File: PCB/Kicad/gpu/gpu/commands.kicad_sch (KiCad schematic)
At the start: 1 part, among them U1 74LS08

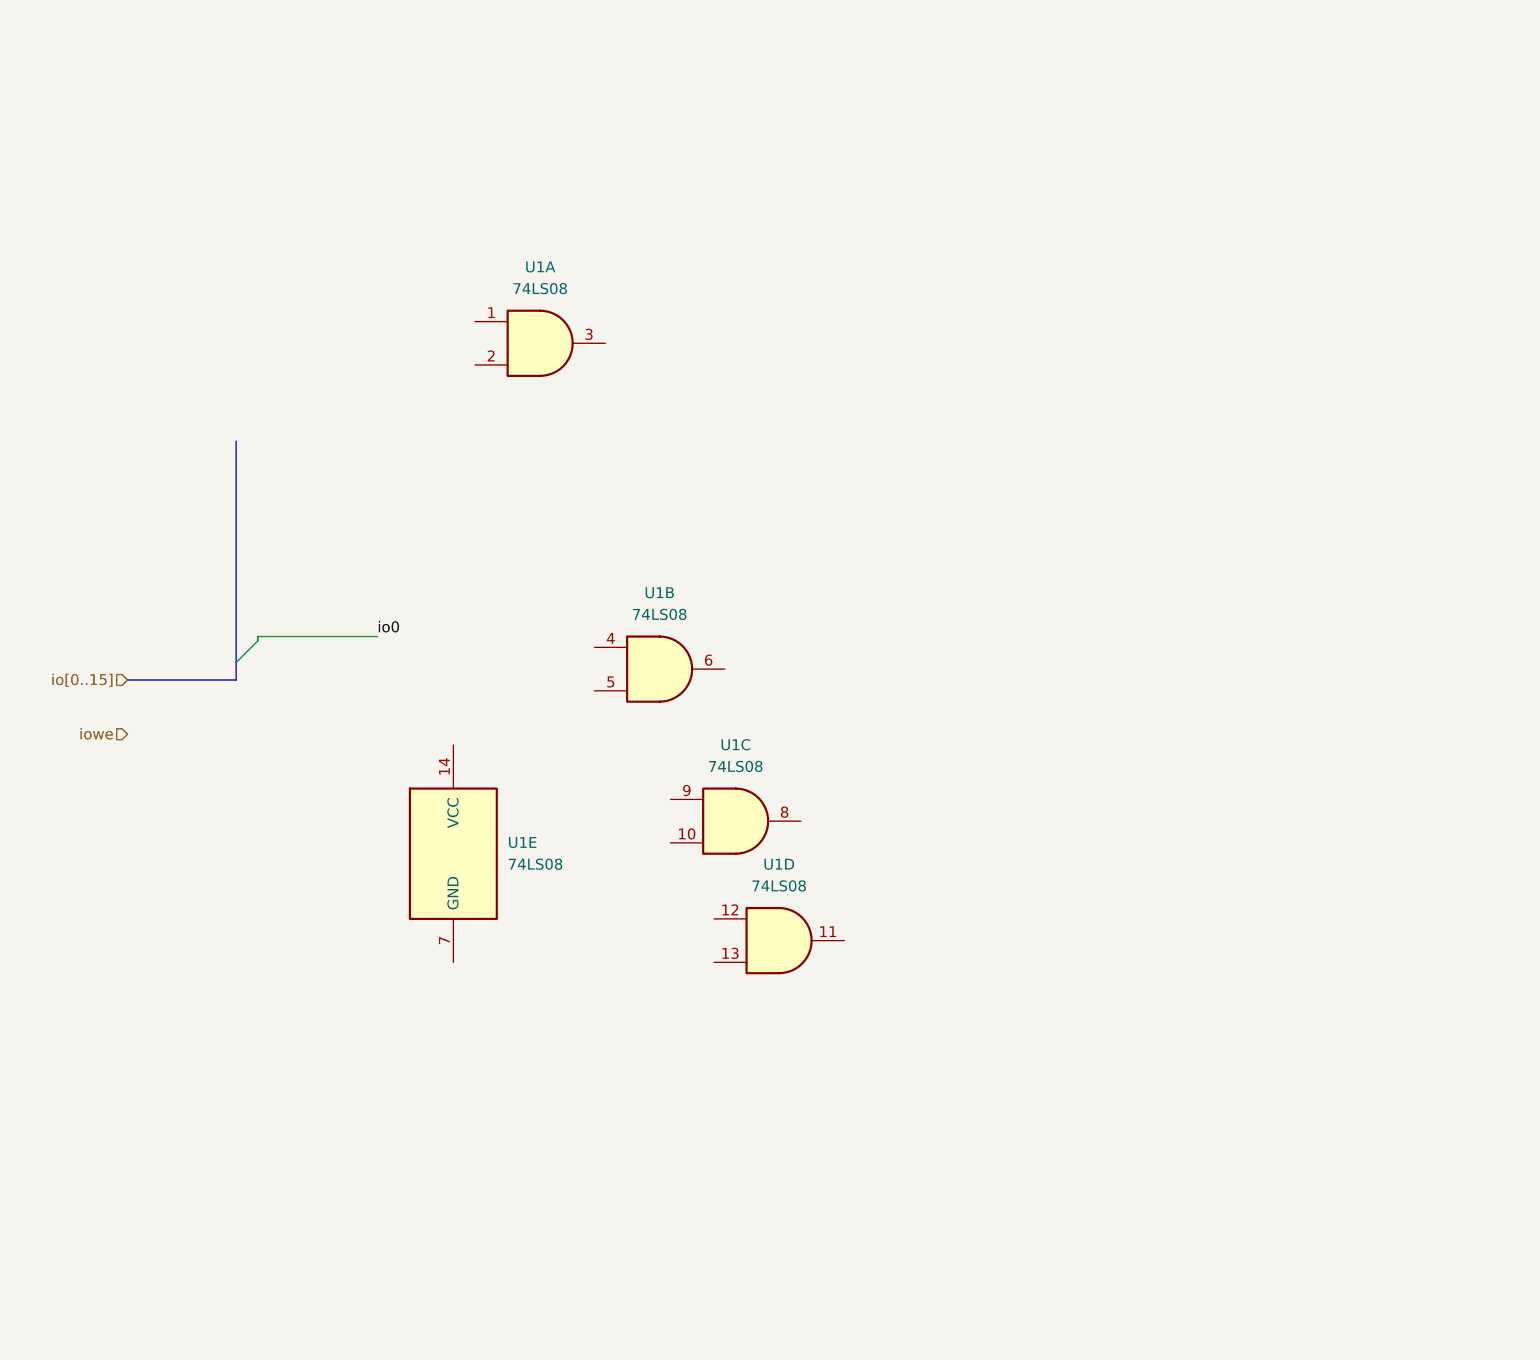
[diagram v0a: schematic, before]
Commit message: Kicad implementation
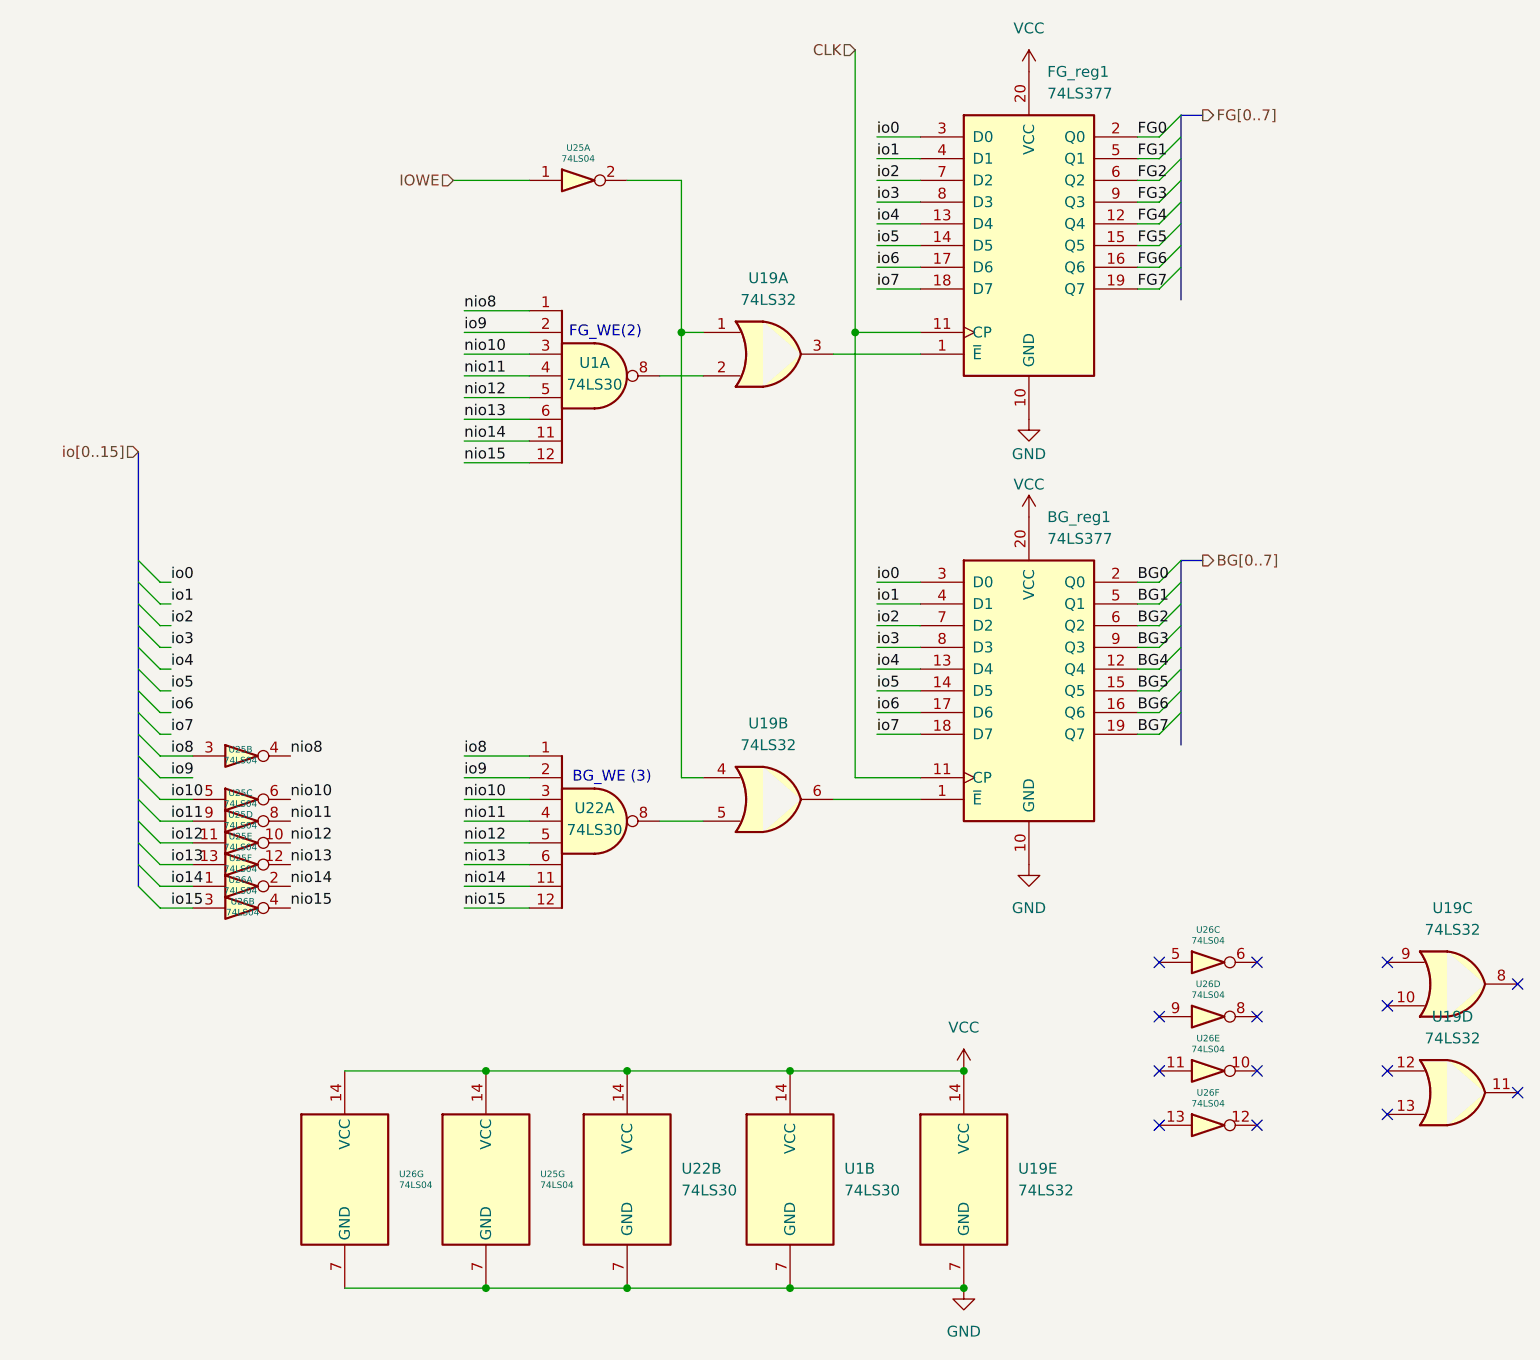
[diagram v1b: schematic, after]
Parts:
- removed U1: 74LS08, symbol 74xx:74LS08
- added BG_reg1, FG_reg1: 74LS377, Package_DIP:DIP-20_W8.89mm_SMDSocket_LongPads, symbol 74xx:74LS377
- added U1, U22: 74LS30, Package_DIP:DIP-14_W8.89mm_SMDSocket_LongPads, symbol 74xx:74LS30
- added U19: 74LS32, Package_DIP:DIP-14_W8.89mm_SMDSocket_LongPads, symbol 74xx:74LS32
- added U25, U26: 74LS04, Package_DIP:DIP-14_W8.89mm_SMDSocket_LongPads, symbol 74xx1:74LS04
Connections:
- net io0: now also BG_reg1.3 (D0), FG_reg1.3 (D0)
- new net: U19.1, U19.4, U25.2
- new net: U19.5, U22.8
- new net: BG_reg1.1 (~{E}), U19.6
- new net: FG_reg1.1 (~{E}), U19.3
- new net: U1.8, U19.2
- new net BG0: BG_reg1.2 (Q0)
- new net BG1: BG_reg1.5 (Q1)
- new net BG2: BG_reg1.6 (Q2)
- new net BG3: BG_reg1.9 (Q3)
- new net BG4: BG_reg1.12 (Q4)
- new net BG5: BG_reg1.15 (Q5)
- new net BG6: BG_reg1.16 (Q6)
- new net BG7: BG_reg1.19 (Q7)
- new net CLK: BG_reg1.11 (CP), FG_reg1.11 (CP)
- new net FG0: FG_reg1.2 (Q0)
- new net FG1: FG_reg1.5 (Q1)
- new net FG2: FG_reg1.6 (Q2)
- new net FG3: FG_reg1.9 (Q3)
- new net FG4: FG_reg1.12 (Q4)
- new net FG5: FG_reg1.15 (Q5)
- new net FG6: FG_reg1.16 (Q6)
- new net FG7: FG_reg1.19 (Q7)
- new net GND: BG_reg1.10 (GND), FG_reg1.10 (GND), U1.7 (GND), U19.7 (GND), U22.7 (GND), U25.7 (GND), U26.7 (GND)
- new net IOWE: U25.1
- new net VCC: BG_reg1.20 (VCC), FG_reg1.20 (VCC), U1.14 (VCC), U19.14 (VCC), U22.14 (VCC), U25.14 (VCC), U26.14 (VCC)
- new net io1: BG_reg1.4 (D1), FG_reg1.4 (D1)
- new net io10: U25.5
- new net io11: U25.9
- new net io12: U25.11
- new net io13: U25.13
- new net io14: U26.1
- new net io15: U26.3
- new net io2: BG_reg1.7 (D2), FG_reg1.7 (D2)
- new net io3: BG_reg1.8 (D3), FG_reg1.8 (D3)
- new net io4: BG_reg1.13 (D4), FG_reg1.13 (D4)
- new net io5: BG_reg1.14 (D5), FG_reg1.14 (D5)
- new net io6: BG_reg1.17 (D6), FG_reg1.17 (D6)
- new net io7: BG_reg1.18 (D7), FG_reg1.18 (D7)
- new net io8: U22.1, U25.3
- new net io9: U1.2, U22.2
- new net nio10: U1.3, U22.3, U25.6
- new net nio11: U1.4, U22.4, U25.8
- new net nio12: U1.5, U22.5, U25.10
- new net nio13: U1.6, U22.6, U25.12
- new net nio14: U1.11, U22.11, U26.2
- new net nio15: U1.12, U22.12, U26.4
- new net nio8: U1.1, U25.4
- no-connect marks 0 -> 14
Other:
- note added: "BG_WE (3)"
- note added: "FG_WE(2)"
